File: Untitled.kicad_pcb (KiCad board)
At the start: 2 copper layers, 8.2 x 25.1 mm, 3 parts, among them J1 USB_C_Receptacle_PowerOnly_6P

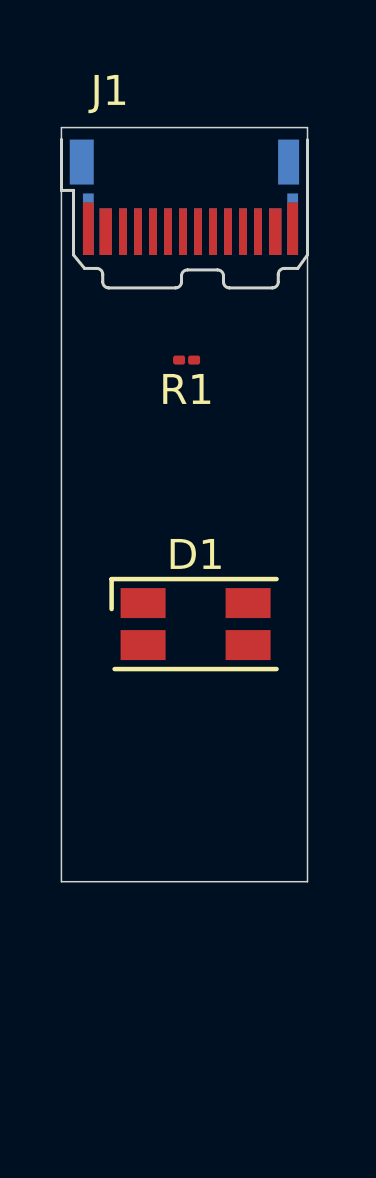
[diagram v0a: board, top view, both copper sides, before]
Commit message: FINSIHEDDD
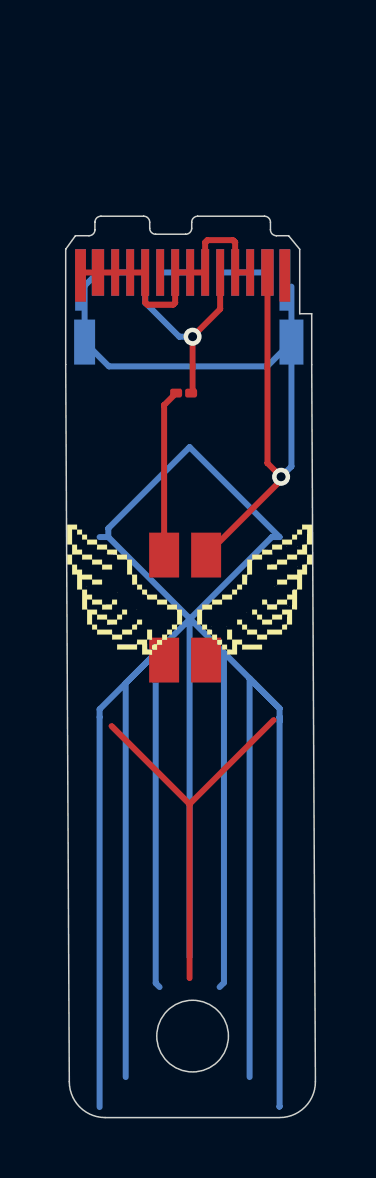
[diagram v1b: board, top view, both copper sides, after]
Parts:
- removed J1: USB_C_Receptacle_PowerOnly_6P, Connector_USB:USB_C_Plug_JAE_DX07P024AJ1
- added G***: LOGO, LOGO, F.Cu at (167.0, 156.0)
- added G***: LOGO, LOGO, B.Cu at (167.0, 156.0)
- added J2: USB_C_Receptacle_PowerOnly_6P, Connector_USB:USB_C_Plug_smaller, F.Cu at (166.8, 146.3)
- moved R1 1.10 mm to (166.8, 149.2)
- moved D1 0.65 mm to (166.8, 156.3), turned to -90 degrees
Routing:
- net (no net): track 0.00 -> 141.1 mm
- net Net-(D1-K): track 0.00 -> 27.8 mm, vias 0 -> 1
- net Net-(J2-VBUS-PadA9): track 0.00 -> 7.48 mm, vias 0 -> 1
- net Net-(D1-A): track 0.00 -> 5.57 mm
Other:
- board size 8.2 x 25.1 mm -> 8.3 x 25.1 mm
